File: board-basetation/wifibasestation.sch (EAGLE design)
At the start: 33 parts, among them IC1 1117EMP, IC2 STM32F072, IC3 HTU21D, J1 SWD_SHROUD_SMD, X1 ESP-03, X2 SMA-142-0711-821/826

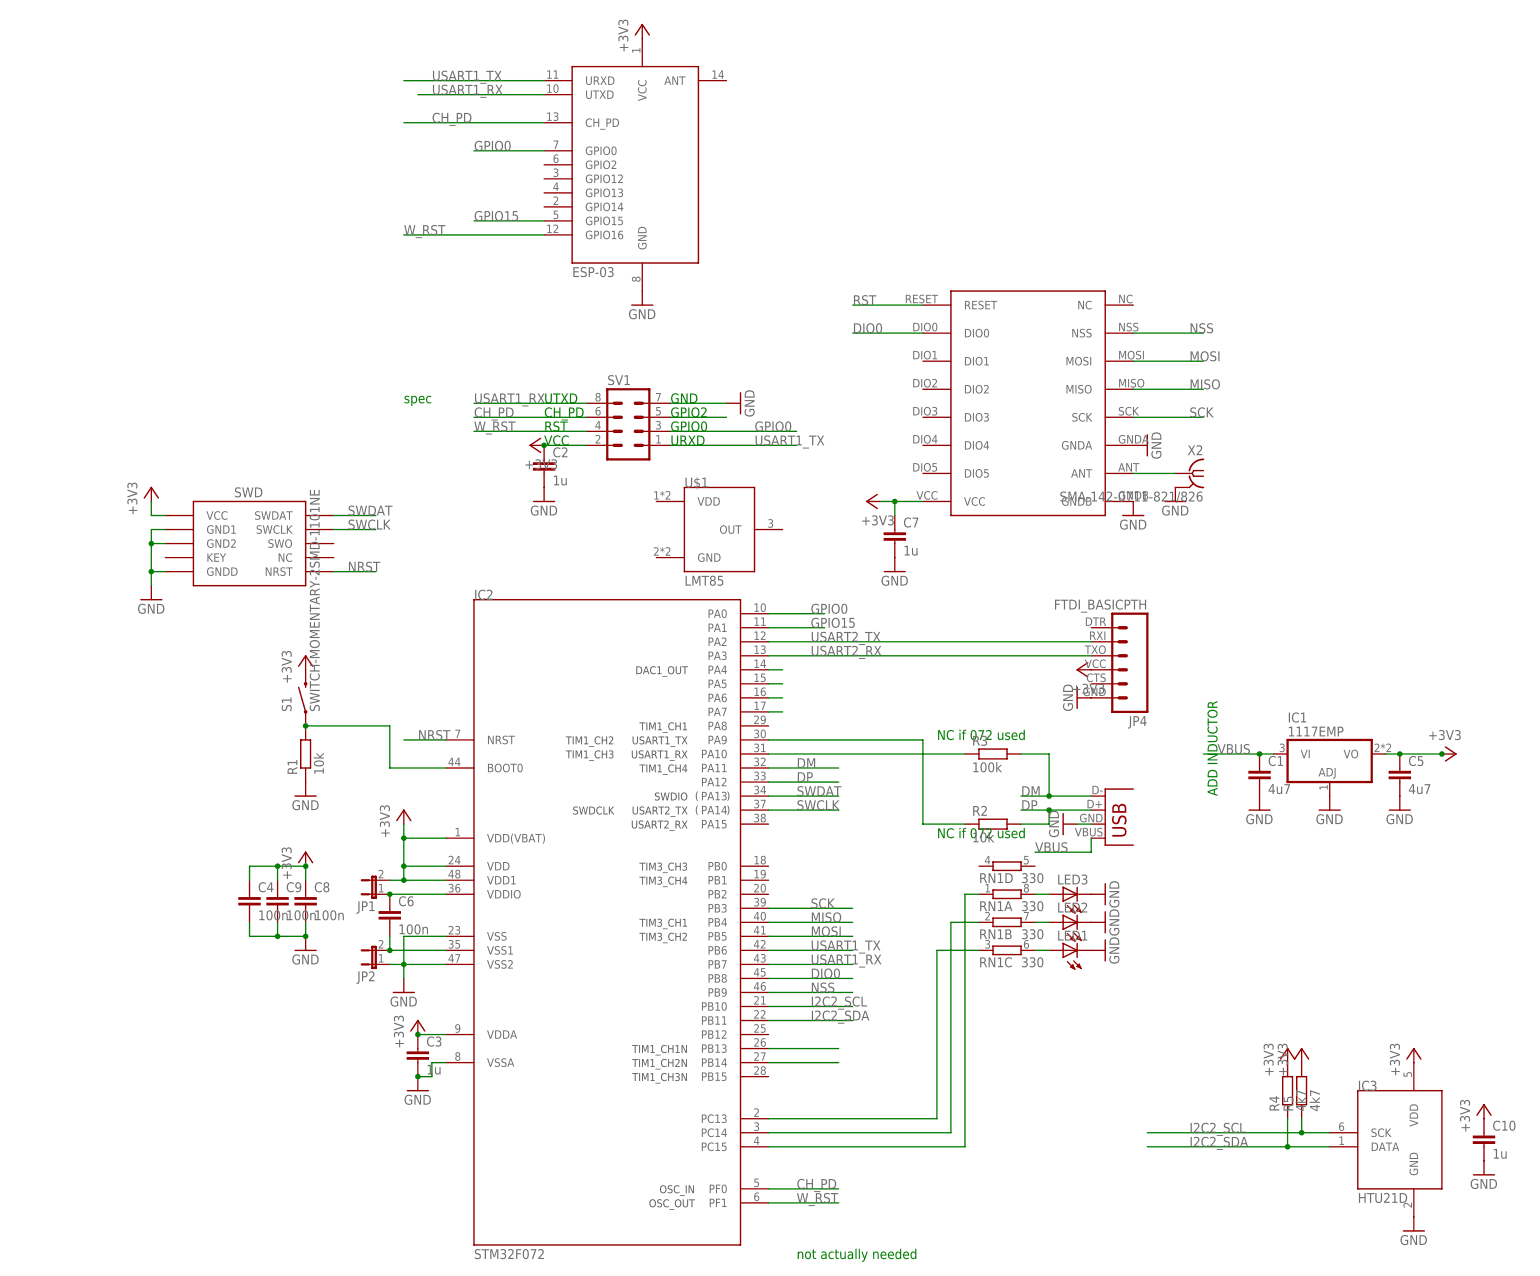
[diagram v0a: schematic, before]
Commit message: almost done
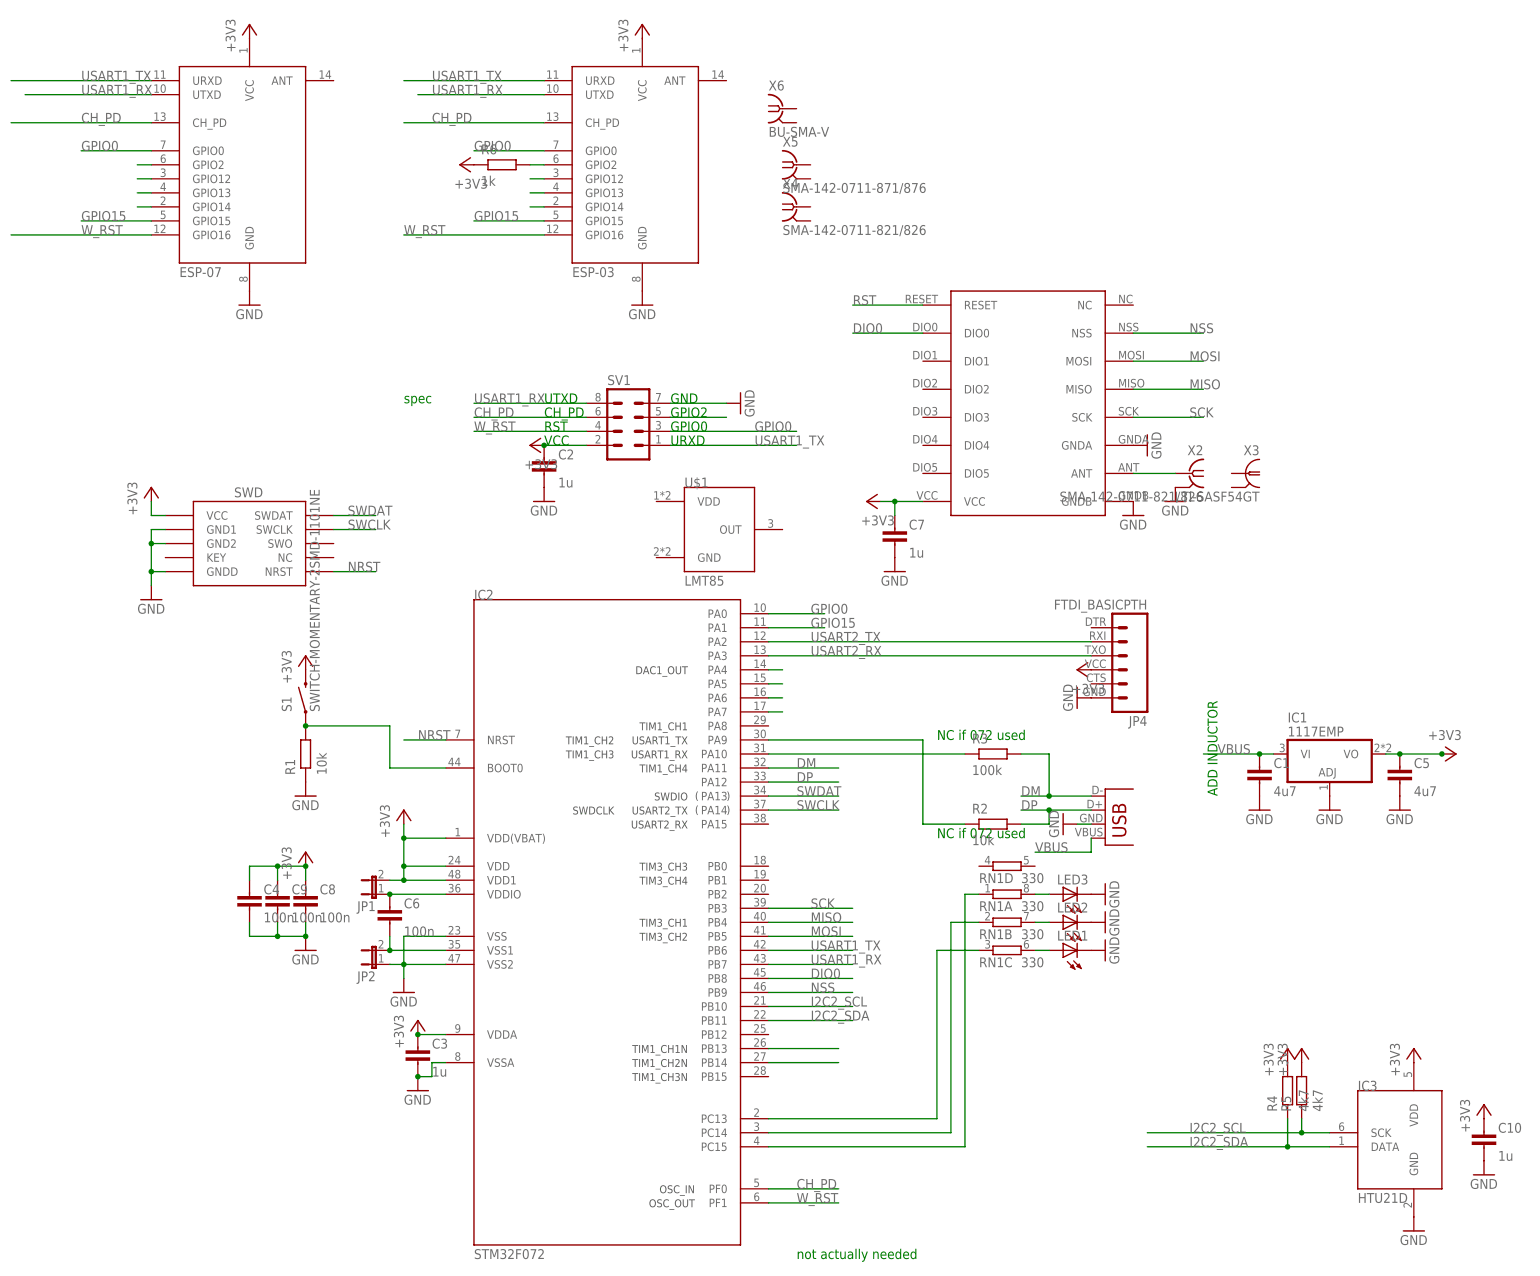
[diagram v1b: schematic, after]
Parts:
- added R6: 1k, passives-7351:RESISTOR0603-N
- added U$3: ESP-07, Mine:ESP-07
- added X3: LTI-SASF54GT, con-coax:LTI-SASF54GT
- added X4: SMA-142-0711-821/826, con-coax:SMA-142-0711-821/826
- added X5: SMA-142-0711-871/876, con-coax:SMA-142-0711-871/876
- added X6: BU-SMA-V, con-coax:BU-SMA-V
- C1, C10, C2, C3, C4, C7, C8, C9: device rcl:C-EUC0603 -> passives-7351:CAPACITOR0603-N
- C5: device rcl:C-EUC0805 -> passives-7351:CAPACITOR0805-N
- C6: device rcl:C-EUC0603K -> passives-7351:CAPACITOR0603-N
- R1, R2, R3, R4, R5: device rcl:R-EU_R0603 -> passives-7351:RESISTOR0603-N
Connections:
- new net N$1: R6.P$2, U$3.GPIO2, X1.GPIO2
- new net N$3: U$3.GPIO14, X1.GPIO14
- new net N$4: U$3.GPIO13, X1.GPIO13
- new net N$7: U$3.GPIO12, X1.GPIO12
- net +3V3: now also R4.P$2, R5.P$2, R6.P$1, U$3.VCC; no longer R4.2, R5.2
- net CH_PD: now also U$3.CH_PD
- net DM: now also R3.P$2; no longer R3.2
- net DP: now also R2.P$2; no longer R2.2
- net GND: now also R1.P$1, U$3.GND; no longer R1.1
- net GPIO0: now also U$3.GPIO0
- net GPIO15: now also U$3.GPIO15
- net I2C2_SCL: now also R5.P$1; no longer R5.1
- net I2C2_SDA: now also R4.P$1; no longer R4.1
- net N$15: now also R1.P$2; no longer R1.2
- net N$17: now also R3.P$1; no longer R3.1
- net N$18: now also R2.P$1; no longer R2.1
- net USART1_RX: now also U$3.UTXD
- net USART1_TX: now also U$3.URXD
- net W_RST: now also U$3.GPIO16
